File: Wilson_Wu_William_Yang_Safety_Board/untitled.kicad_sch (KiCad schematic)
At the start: 29 parts, among them J18 XT60-M, J3 430450200, J5 430450200, J6 XT60-M, J7 XT60-M, Q1 IRLML6344TRPBF, Q2 IRLML6344TRPBF, U12 J115F11AH12VDCS61.5U, U16 J115F11AH12VDCS61.5U, U5 J115F11AH12VDCS61.5U, U6 J115F11AH12VDCS61.5U

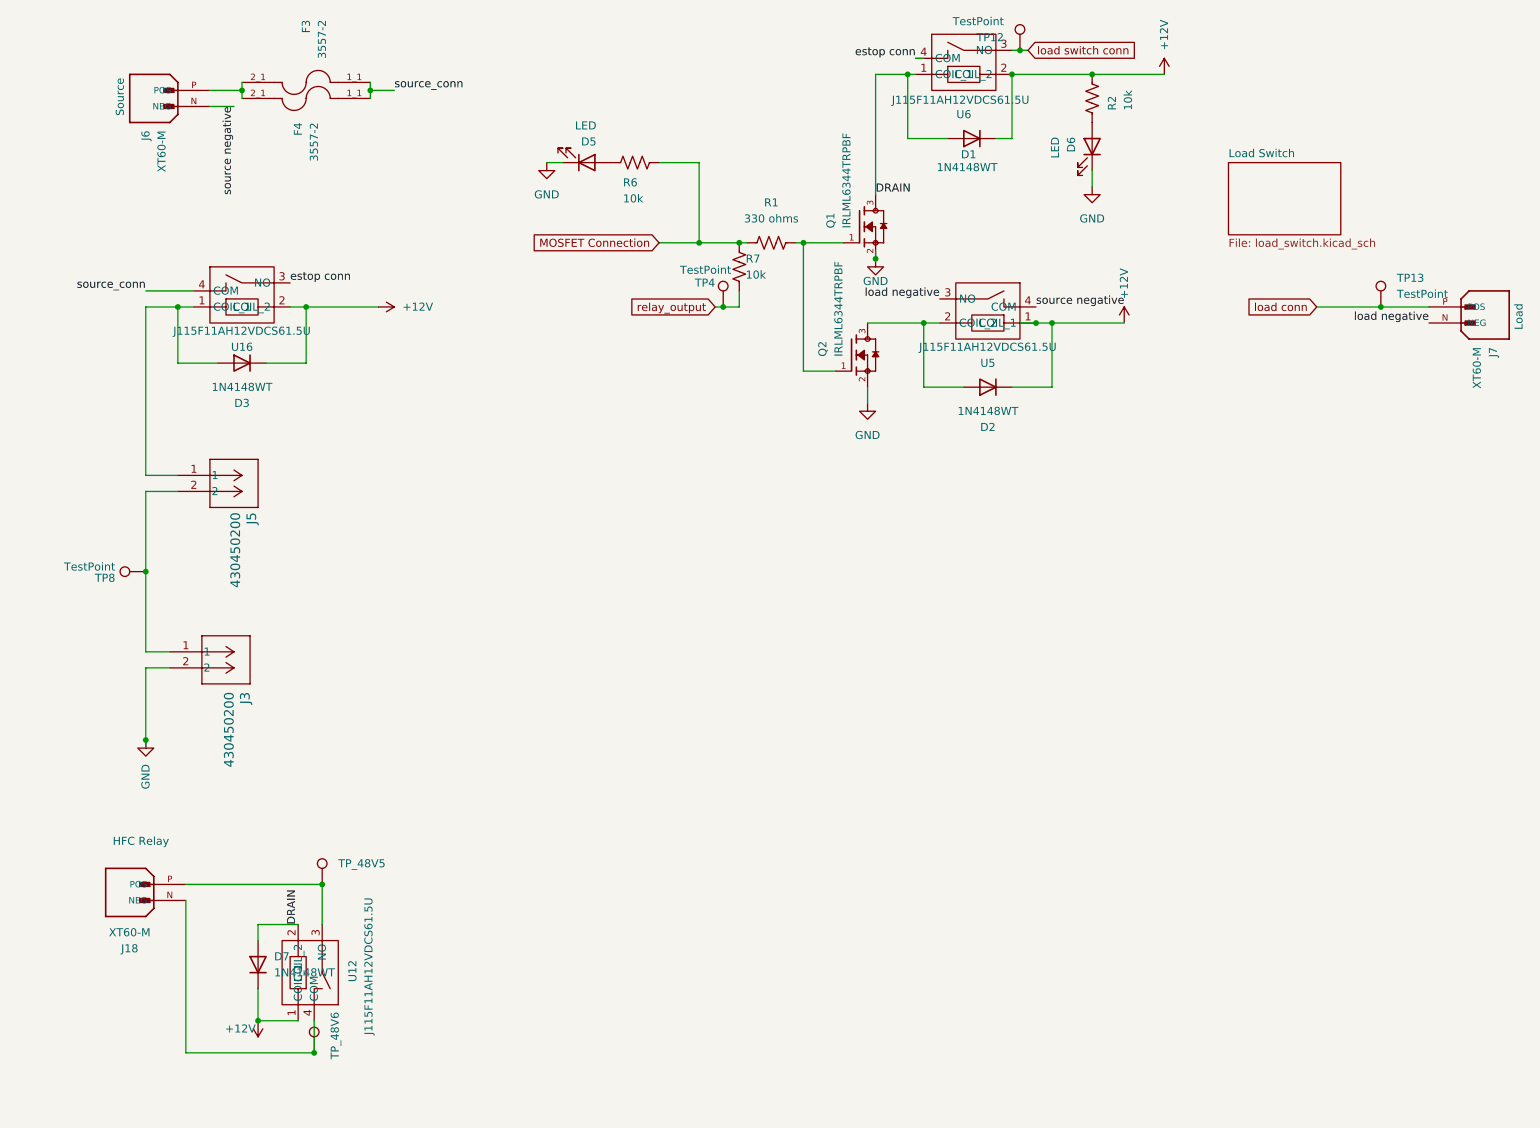
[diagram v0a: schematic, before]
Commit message: comp placement
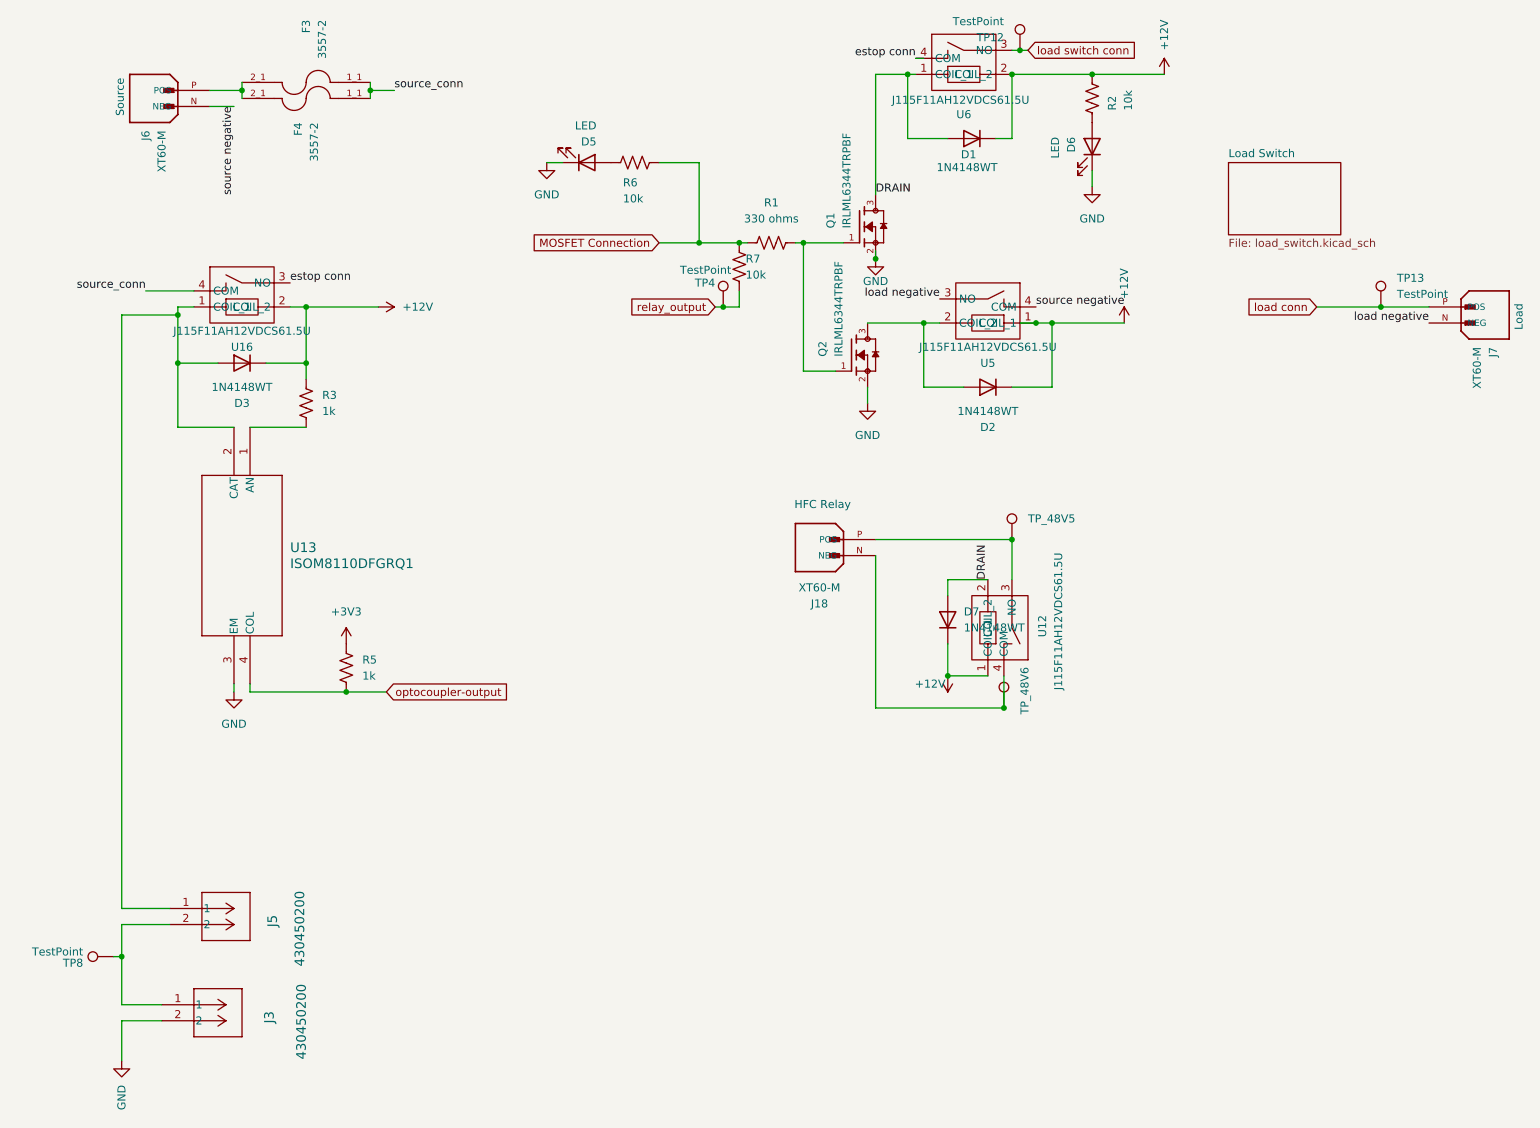
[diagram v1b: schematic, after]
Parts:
- added R3, R5: 1k, SMV_Passives:0603_resistors, symbol Device:R_US
- added U13: ISOM8110DFGRQ1, octocoupler:DFG0004A_TEX, symbol octocoupler:ISOM8110DFGRQ1
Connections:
- net +12V: now also R3.1
- net GND: now also U13.3 (EM)
- net at D3.2 (A), J5.1, U16.1 (COIL_1): now also U13.2 (CAT)
- new net: R3.2, U13.1 (AN)
- new net +3V3: R5.1
- new net optocoupler-output: R5.2, U13.4 (COL)
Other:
- moved on the sheet: D7, J18, J3, J5, TP8, TP_48V5, TP_48V6, U12

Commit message: bruh
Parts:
- TP12, TP13: footprint TestPoint:TestPoint_Loop_D2.54mm_Drill1.5mm_Beaded -> TestPoint:TestPoint_Pad_D1.0mm
- TP_48V5, TP_48V6: footprint TestPoint:TestPoint_Pad_D2.0mm -> TestPoint:TestPoint_Pad_D1.0mm
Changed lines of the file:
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@@
 			)
 		)
-		(property "Footprint" "TestPoint:TestPoint_Loop_D2.54mm_Drill1.5mm_Beaded"
+		(property "Footprint" "TestPoint:TestPoint_Pad_D1.0mm"
 			(at 170.18 27.94 0)
 			(effects
@@
 			)
 		)
-		(property "Footprint" "TestPoint:TestPoint_Loop_D2.54mm_Drill1.5mm_Beaded"
+		(property "Footprint" "TestPoint:TestPoint_Pad_D1.0mm"
 			(at 227.33 68.58 0)
 			(effects
@@
 			)
 		)
-		(property "Footprint" "TestPoint:TestPoint_Pad_D2.0mm"
+		(property "Footprint" "TestPoint:TestPoint_Pad_D1.0mm"
 			(at 168.91 105.41 0)
 			(effects
@@
 			)
 		)
-		(property "Footprint" "TestPoint:TestPoint_Pad_D2.0mm"
+		(property "Footprint" "TestPoint:TestPoint_Pad_D1.0mm"
 			(at 167.64 132.08 0)
 			(effects
